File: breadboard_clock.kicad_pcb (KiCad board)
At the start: 2 copper layers, 102.1 x 29.3 mm, 34 parts, among them J1 Conn_01x02_Male, J2 Conn_01x03_Male, P1 R_POT, SW1 SW_Push, SW2 SW_SPDT, U1 ICM7555, U2 74LS04, U3 74LS04, U4 74LS08, U5 ICM7555, U6 74LS32, U7 74LS04, U8 ICM7555

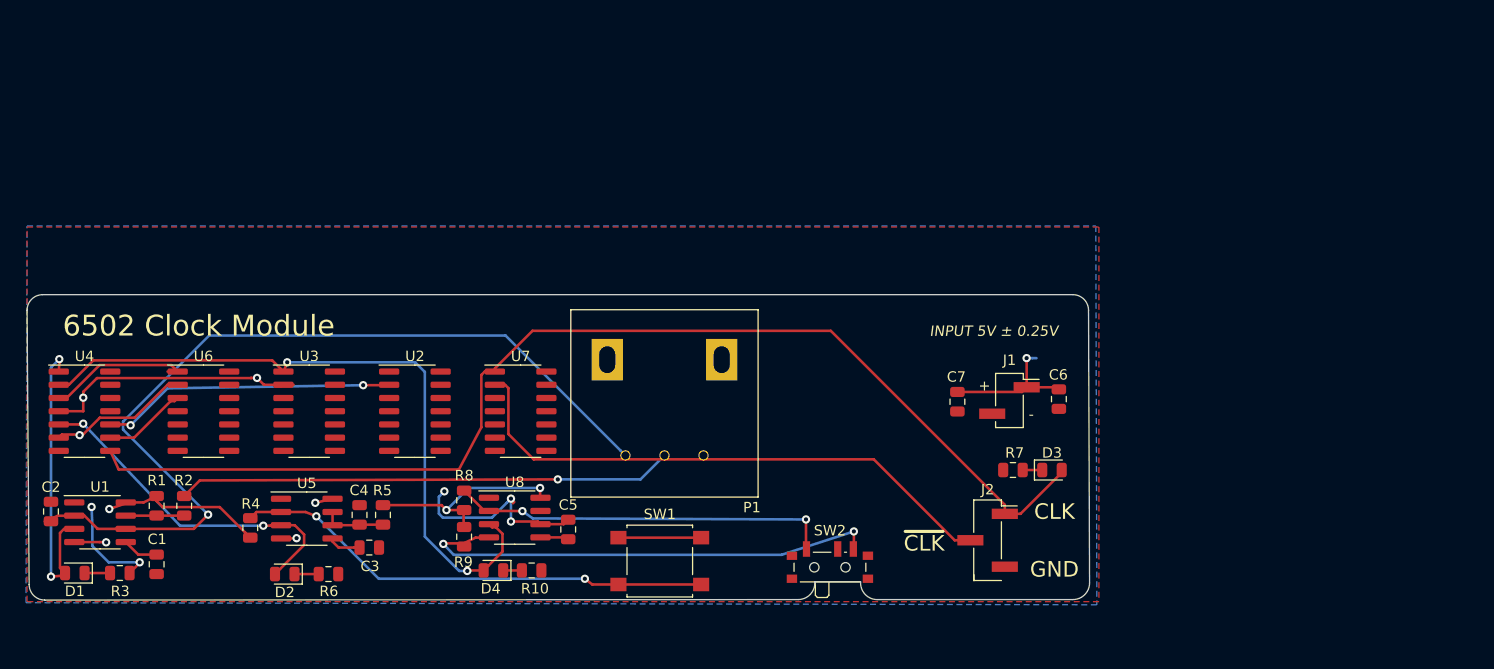
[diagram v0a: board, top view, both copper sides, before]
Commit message: Add files via upload
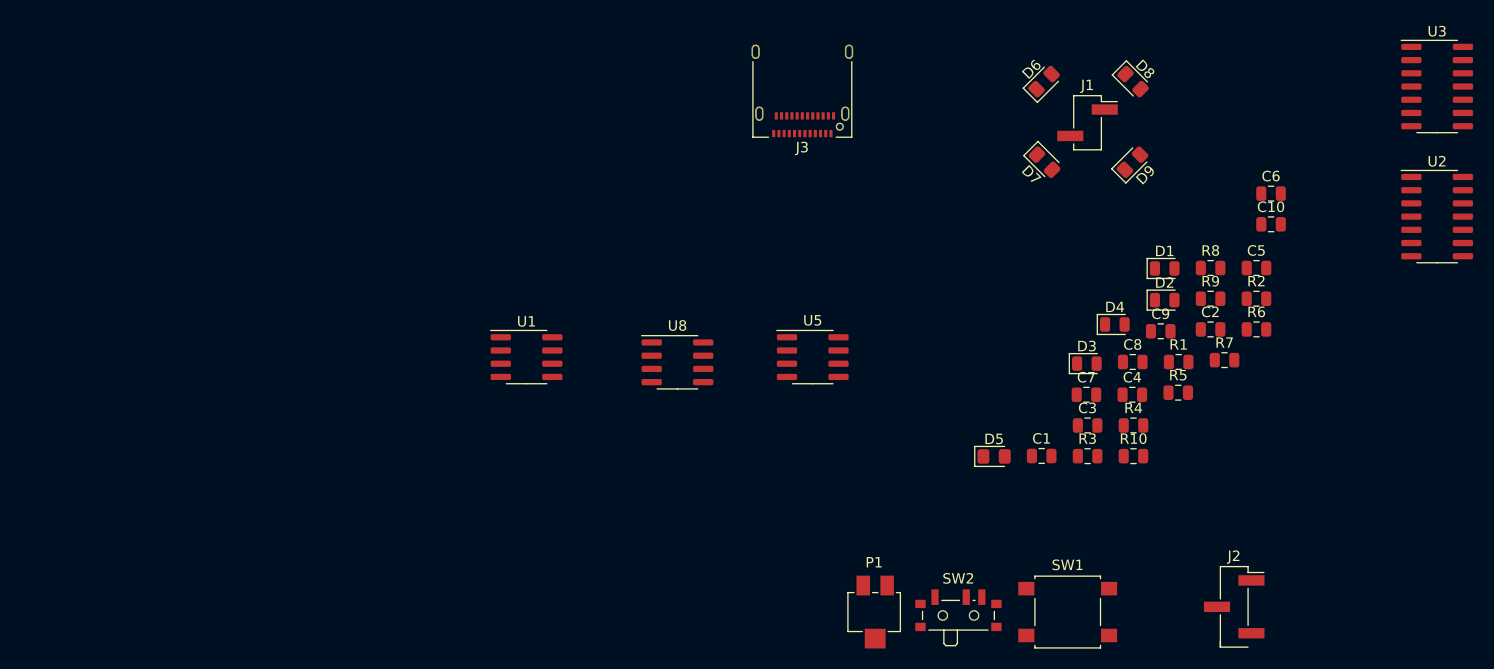
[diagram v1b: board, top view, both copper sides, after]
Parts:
- removed U4: 74LS08, Package_SO:SOIC-14_3.9x8.7mm_P1.27mm
- removed U6: 74LS32, Package_SO:SOIC-14_3.9x8.7mm_P1.27mm
- removed U7: 74LS04, Package_SO:SOIC-14_3.9x8.7mm_P1.27mm
- added C10: 0.1uF, Capacitor_SMD:C_0805_2012Metric, F.Cu at (157.5, 80.7)
- added C8: 0.1uF, Capacitor_SMD:C_0805_2012Metric, F.Cu at (144.2, 94.0)
- added C9: 0.1uF, Capacitor_SMD:C_0805_2012Metric, F.Cu at (146.9, 91.0)
- added D5: D_Schottky, Diode_SMD:D_0805_2012Metric_Pad1.15x1.40mm_HandSolder, F.Cu at (130.9, 103.0)
- added D6: D_Schottky, Diode_SMD:D_0805_2012Metric_Pad1.15x1.40mm_HandSolder, F.Cu at (135.7, 67.0)
- added D7: D_Schottky, Diode_SMD:D_0805_2012Metric_Pad1.15x1.40mm_HandSolder, F.Cu at (135.8, 74.8)
- added D8: D_Schottky, Diode_SMD:D_0805_2012Metric_Pad1.15x1.40mm_HandSolder, F.Cu at (144.3, 67.0)
- added D9: D_Schottky, Diode_SMD:D_0805_2012Metric_Pad1.15x1.40mm_HandSolder, F.Cu at (144.2, 74.8)
- added J3: USB_C_Receptacle_USB2.0, Connector_USB:USB_C_Receptacle_Amphenol_12401610E4-2A, F.Cu at (112.5, 67.0)
- C7: value 0.1uF -> 1uF
- P1: value R_POT -> 1M; footprint Gerig-Added:Potentiomter_Bourns_PDB12_THT -> Potentiometer_SMD:Potentiometer_Bourns_3224X_Vertical
- U2: value 74LS04 -> 74LS04-Full
- U3: value 74LS04 -> 74LS08-Full
- moved C2 112.8 mm to (151.7, 90.8), turned to 0 degrees
- moved U3 112.8 mm to (173.5, 67.5)
- moved D1 108.7 mm to (147.3, 85.0), turned to 0 degrees
- moved R2 104.9 mm to (156.1, 87.9), turned to 0 degrees
- moved U2 100.0 mm to (173.5, 80.0)
- moved R1 99.2 mm to (148.7, 94.0), turned to 0 degrees
- moved R3 93.7 mm to (139.9, 103.0)
- moved R6 92.2 mm to (156.1, 90.8)
- moved D2 88.6 mm to (147.3, 88.0), turned to 0 degrees
- moved C1 85.7 mm to (135.5, 103.0), turned to 0 degrees
- moved R4 85.4 mm to (144.3, 100.1), turned to 0 degrees
- moved R5 77.3 mm to (148.6, 96.9), turned to 0 degrees
- moved R9 75.3 mm to (151.7, 87.9), turned to 0 degrees
- moved C4 75.2 mm to (144.2, 97.1), turned to 0 degrees
- moved R8 75.1 mm to (151.7, 84.9), turned to 0 degrees
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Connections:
- J1 pad 1: VCC -> PowerSupply-
- J1 pad 2: GND -> PowerSupply+
- J2 pad 1: CLK -> ~CLK
- J2 pad 2: ~CLK -> CLK
- R9 pad 2: Net-(R9-Pad2) -> GND
- SW2 pad 3: Net-(R9-Pad2) -> GND
- U2 pad 1: HALT -> Net-(D4-Pad2)
- U2 pad 10: (no net) -> CLK
- U2 pad 11: (no net) -> Net-(U2-Pad11)
- U2 pad 12: (no net) -> ~CLK
- U2 pad 13: (no net) -> CLK
- U2 pad 14: (no net) -> VCC
- U2 pad 3: (no net) -> Net-(U2-Pad3)
- U2 pad 4: (no net) -> Net-(U2-Pad4)
- U2 pad 5: (no net) -> Net-(U2-Pad5)
- U2 pad 6: (no net) -> Net-(U2-Pad6)
- U2 pad 7: (no net) -> GND
- U2 pad 8: (no net) -> Net-(U2-Pad8)
- U2 pad 9: (no net) -> GND
- U3 pad 1: Net-(D4-Pad2) -> Net-(D1-Pad2)
- U3 pad 10: (no net) -> GND
- U3 pad 11: (no net) -> Net-(U2-Pad11)
- U3 pad 12: (no net) -> Net-(U2-Pad4)
- U3 pad 13: (no net) -> Net-(U2-Pad6)
- U3 pad 14: (no net) -> VCC
- U3 pad 2: Net-(U3-Pad2) -> Net-(D4-Pad2)
- U3 pad 3: (no net) -> Net-(U2-Pad3)
- U3 pad 4: (no net) -> Net-(U2-Pad2)
- U3 pad 5: (no net) -> Net-(D2-Pad2)
- U3 pad 6: (no net) -> Net-(U2-Pad5)
- U3 pad 7: (no net) -> GND
- U3 pad 8: (no net) -> Net-(U3-Pad8)
- U3 pad 9: (no net) -> GND
- U8 pad 4: Net-(R9-Pad2) -> GND
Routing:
- net CLK: track 111.7 -> 0.00 mm
- net Net-(C2-Pad1): track 85.7 -> 0.00 mm, vias 1 -> 0
- net Net-(D4-Pad2): track 66.4 -> 0.00 mm, vias 2 -> 0
- net VCC: track 56.4 -> 0.00 mm, vias 7 -> 0
- net ~CLK: track 54.5 -> 0.00 mm
- net Net-(P1-Pad2): track 47.7 -> 0.00 mm, vias 1 -> 0
- net Net-(R4-Pad2): track 47.3 -> 0.00 mm, vias 2 -> 0
- net Net-(R9-Pad2): track 46.7 -> 0.00 mm, vias 2 -> 0
- net GND: track 36.8 -> 0.00 mm, vias 5 -> 0
- net Net-(R8-Pad2): track 36.7 -> 0.00 mm, vias 2 -> 0
- net Net-(D2-Pad2): track 34.2 -> 0.00 mm, vias 2 -> 0
- net Net-(D1-Pad2): track 29.5 -> 0.00 mm, vias 2 -> 0
- net Net-(U2-Pad2): track 28.4 -> 0.00 mm, vias 2 -> 0
- net Net-(U3-Pad2): track 25.3 -> 0.00 mm, vias 2 -> 0
- net Net-(U4-Pad3): track 14.0 -> 0.00 mm
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- removed copper zone on F.Cu, net GND
- removed copper zone on B.Cu, net VCC
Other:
- board outline removed
- rule pad_to_mask_clearance: 0.051 -> 0
- board text removed: "+"
- board text removed: "-"
- board text removed: "6502 Clock Module"
- board text removed: "CLK"
- board text removed: "GND"
- board text removed: "INPUT 5V ± 0.25V"
- board text removed: "~CLK"
